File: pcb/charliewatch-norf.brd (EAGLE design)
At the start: 30.5 x 30.5 mm, 86 parts, among them U1 LIS3DH, U2 CC430F5137IRGZR, X1 CRYSTALS-NOGND-IQXC-25

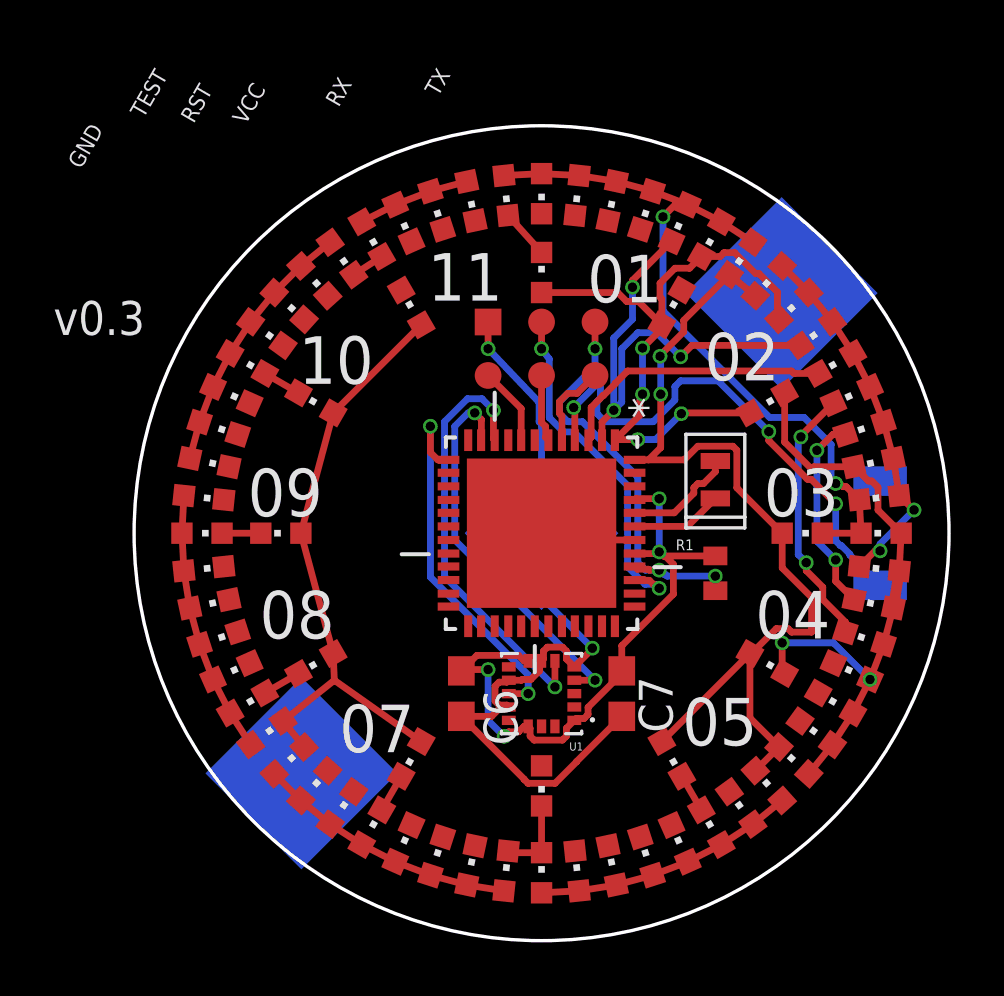
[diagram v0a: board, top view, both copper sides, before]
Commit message: Finish Routing
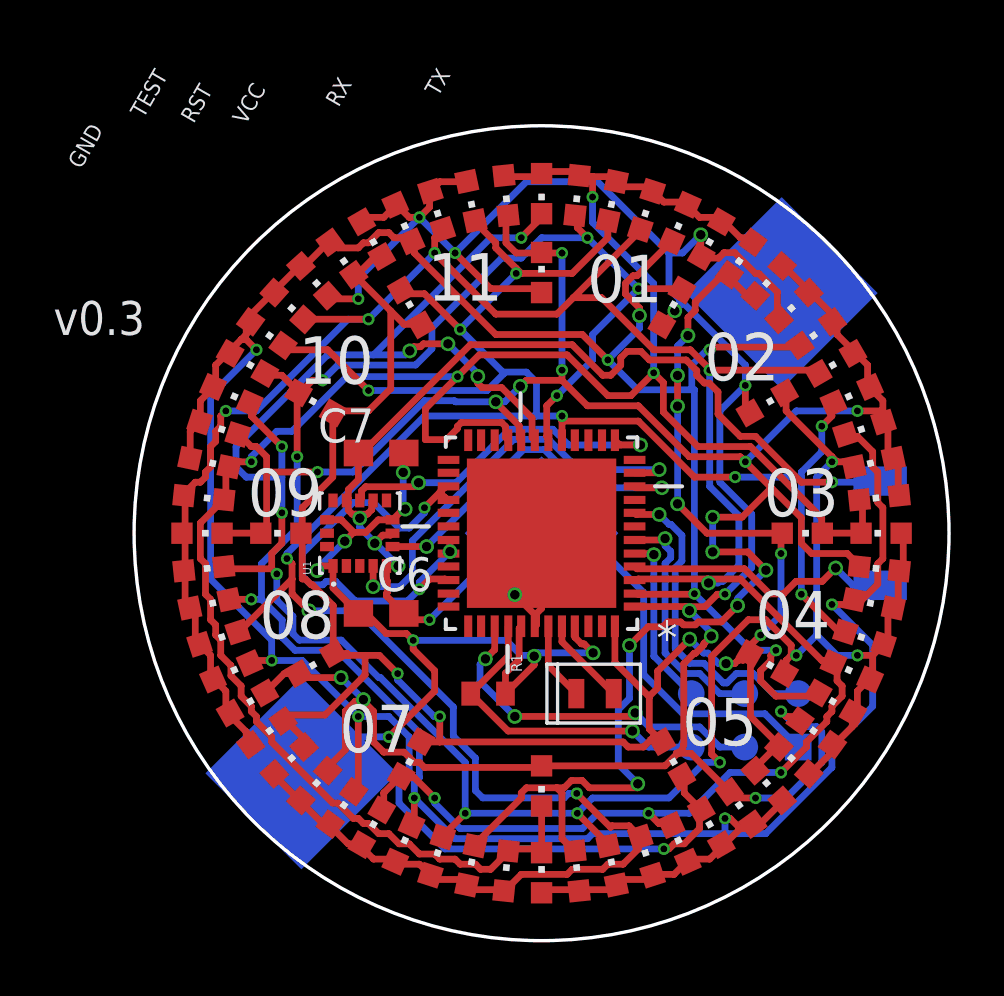
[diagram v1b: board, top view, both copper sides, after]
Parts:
- moved TP1 19.7 mm to (29.6, 12.0), flipped to the bottom
- moved TP5 17.6 mm to (27.6, 12.0), flipped to the bottom
- moved TP2 16.6 mm to (29.6, 14.0), flipped to the bottom
- moved TP6 16.3 mm to (25.6, 12.0), flipped to the bottom
- moved TP3 14.1 mm to (27.6, 14.0), flipped to the bottom
- moved C7 12.7 mm to (14.0, 23.0), turned to 180 degrees
- moved TP4 12.4 mm to (25.6, 14.0), flipped to the bottom
- moved R1 9.62 mm to (18.0, 14.0), turned to 0 degrees
- moved X1 9.18 mm to (22.0, 14.0), turned to 0 degrees
- moved U1 9.07 mm to (13.2, 20.0), turned to 90 degrees
- moved C6 4.24 mm to (14.0, 17.0), turned to 0 degrees
- turned U$1 to 135 degrees
- turned U2 to 180 degrees
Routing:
- net B4: track 19.7 -> 100.0 mm, vias 2 -> 10
- net B3: track 18.8 -> 94.7 mm, vias 2 -> 9
- net B2: track 23.1 -> 95.8 mm, vias 2 -> 13
- net B1: track 17.1 -> 88.0 mm, vias 2 -> 13
- net B5: track 21.9 -> 90.4 mm, vias 0 -> 8
- net B6: track 29.7 -> 97.5 mm, vias 3 -> 9
- net B7: track 29.4 -> 93.1 mm, vias 4 -> 13
- net B0: track 31.2 -> 83.2 mm, vias 2 -> 4
- net GND: track 33.9 -> 63.3 mm, vias 2 -> 6
- net B8: track 58.0 -> 78.3 mm, vias 2 -> 10
- net AVCC: track 0.00 -> 17.4 mm, vias 0 -> 3
- net VCC: track 24.5 -> 34.4 mm, vias 4 -> 8
- net BUTTON: track 19.8 -> 10.3 mm, vias 3 -> 1
- net BSL_VCC: track 2.93 -> 12.1 mm, vias 0 -> 1
- net BSL_RX: track 2.53 -> 9.23 mm, vias 0 -> 1
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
